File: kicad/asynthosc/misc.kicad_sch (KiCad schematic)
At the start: 8 parts, among them J4 LOUT, U4 TL074

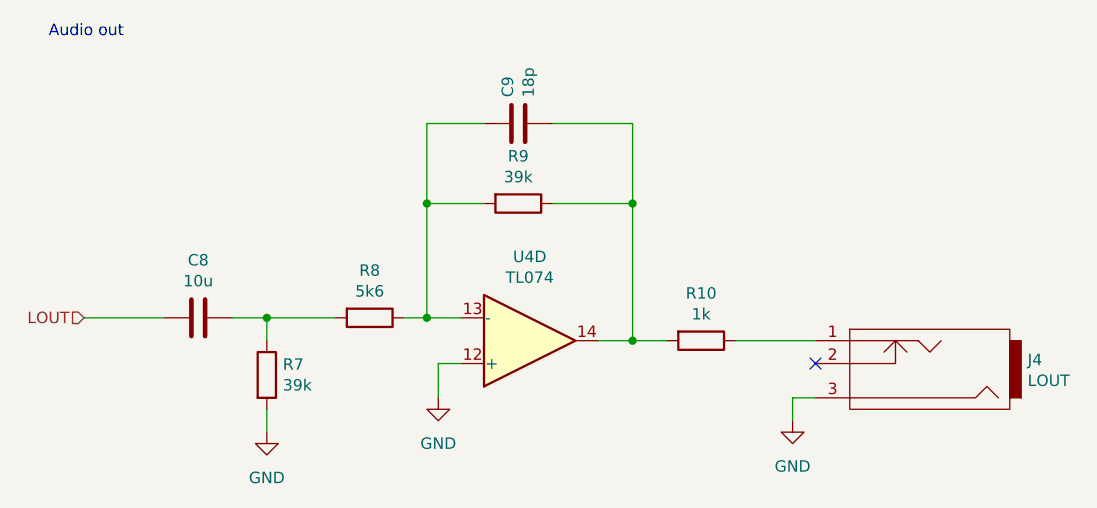
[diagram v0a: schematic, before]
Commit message: sch: wip, add .gitignore
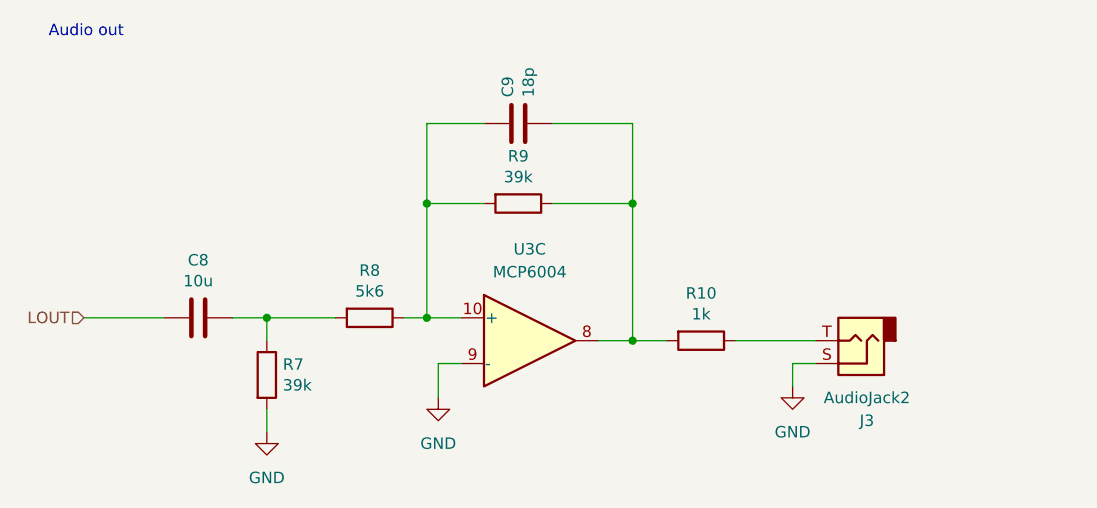
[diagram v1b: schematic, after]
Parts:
- removed J4: LOUT, connectors:THONKICONN, symbol jack_2p:JACK_2P
- removed U4: TL074, Package_SO:TSSOP-14_4.4x5mm_P0.65mm, symbol Amplifier_Operational:TL074
- added J3: AudioJack2, symbol Connector_Audio:AudioJack2
- added U3: MCP6004, symbol Amplifier_Operational:MCP6004
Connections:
- net GND: now also J3.S, U3.9 (-)
- net at C9.2, R10.2, R9.1: now also U3.8
- net at C9.1, R8.1, R9.2: now also U3.10 (+)
- net at R10.1: now also J3.T
- no-connect marks 1 -> 0
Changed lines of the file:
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@@
 		(color 0 0 0 0)
 	)
-	(no_connect
-		(at 115.57 54.61)
-	)
 	(wire
 		(pts
@@
 	(wire
 		(pts
-			(xy 115.57 58.42) (xy 113.03 58.42)
+			(xy 115.57 54.61) (xy 113.03 54.61)
 		)
 		(stroke
@@
 	(wire
 		(pts
-			(xy 113.03 58.42) (xy 113.03 60.96)
+			(xy 113.03 54.61) (xy 113.03 57.15)
 		)
 		(stroke
@@
 	)
 	(symbol
-		(lib_id "jack_2p:JACK_2P")
-		(at 127 54.61 180)
-		(unit 1)
-		(exclude_from_sim no)
-		(in_bom yes)
-		(on_board yes)
-		(dnp no)
-		(property "Reference" "J4"
-			(at 139.1412 54.2036 0)
-			(effects
-				(font
-					(size 1.27 1.27)
-				)
-				(justify right)
-			)
-		)
-		(property "Value" "LOUT"
-			(at 139.1412 56.515 0)
-			(effects
-				(font
-					(size 1.27 1.27)
-				)
-				(justify right)
-			)
-		)
-		(property "Footprint" "connectors:THONKICONN"
-			(at 127 54.61 0)
-			(effects
-				(font
-					(size 1.27 1.27)
-				)
-				(hide yes)
-			)
-		)
-		(property "Datasheet" ""
-			(at 127 54.61 0)
-			(effects
-				(font
-					(size 1.27 1.27)
-				)
-			)
-		)
-		(property "Description" ""
-			(at 127 54.61 0)
-			(effects
-				(font
-					(size 1.27 1.27)
-				)
-				(hide yes)
-			)
-		)
-		(pin "1"
-		)
-		(pin "2"
-		)
-		(pin "3"
-		)
-		(instances
-			(project "asynthosc"
-				(path "/d73e377a-a016-415f-8824-91cc6e4907b9/7d8430fa-40d5-422d-97f7-702a1a4b7211"
-					(reference "J4")
-					(unit 1)
-				)
-			)
-		)
-	)
-	(symbol
 		(lib_id "Device:R")
 		(at 102.87 52.07 270)
@@
 	(symbol
 		(lib_id "power:GND")
-		(at 113.03 60.96 0)
+		(at 113.03 57.15 0)
 		(unit 1)
 		(exclude_from_sim no)
@@
 		(fields_autoplaced yes)
 		(property "Reference" "#PWR025"
-			(at 113.03 67.31 0)
+			(at 113.03 63.5 0)
 			(effects
 				(font
@@
 		)
 		(property "Value" "GND"
-			(at 113.03 66.04 0)
+			(at 113.03 62.23 0)
 			(effects
 				(font
@@
 		)
 		(property "Footprint" ""
-			(at 113.03 60.96 0)
+			(at 113.03 57.15 0)
 			(effects
 				(font
@@
 		)
 		(property "Datasheet" ""
-			(at 113.03 60.96 0)
+			(at 113.03 57.15 0)
 			(effects
 				(font
@@
 		)
 		(property "Description" "Power symbol creates a global label with name \"GND\" , ground"
-			(at 113.03 60.96 0)
+			(at 113.03 57.15 0)
 			(effects
 				(font
@@
 	)
 	(symbol
+		(lib_id "Connector_Audio:AudioJack2")
+		(at 120.65 52.07 180)
+		(unit 1)
+		(exclude_from_sim no)
+		(in_bom yes)
+		(on_board yes)
+		(dnp no)
+		(property "Reference" "J3"
+			(at 121.285 60.96 0)
+			(effects
+				(font
+					(size 1.27 1.27)
+				)
+			)
+		)
+		(property "Value" "AudioJack2"
+			(at 121.285 58.42 0)
+			(effects
+				(font
+					(size 1.27 1.27)
+				)
+			)
+		)
+		(property "Footprint" ""
+			(at 120.65 52.07 0)
+			(effects
+				(font
+					(size 1.27 1.27)
+				)
+				(hide yes)
+			)
+		)
+		(property "Datasheet" "~"
+			(at 120.65 52.07 0)
+			(effects
+				(font
+					(size 1.27 1.27)
+				)
+				(hide yes)
+			)
+		)
+		(property "Description" "Audio Jack, 2 Poles (Mono / TS)"
+			(at 120.65 52.07 0)
+			(effects
+				(font
+					(size 1.27 1.27)
+				)
+				(hide yes)
+			)
+		)
+		(property "Sim.Device" "V"
+			(at 120.65 52.07 0)
+			(effects
+				(font
+					(size 1.27 1.27)
+				)
+				(hide yes)
+			)
+		)
+		(property "Sim.Type" "SIN"
+			(at 120.65 52.07 0)
+			(effects
+				(font
+					(size 1.27 1.27)
+				)
+				(hide yes)
+			)
+		)
+		(property "Sim.Pins" "S=- T=+"
+			(at 120.65 52.07 0)
+			(effects
+				(font
+					(size 1.27 1.27)
+				)
+				(hide yes)
+			)
+		)
+		(property "Sim.Params" "dc=0 ampl=0 f=1 td=0 theta=0 phase=0 ac=5"
+			(at 120.65 52.07 0)
+			(effects
+				(font
+					(size 1.27 1.27)
+				)
+				(hide yes)
+			)
+		)
+		(pin "S"
+		)
+		(pin "T"
+		)
+		(instances
+			(project "asynthosc"
+				(path "/d73e377a-a016-415f-8824-91cc6e4907b9/7d8430fa-40d5-422d-97f7-702a1a4b7211"
+					(reference "J3")
+					(unit 1)
+				)
+			)
+		)
+	)
+	(symbol
 		(lib_id "Device:R")
 		(at 66.04 49.53 270)
@@
 	)
 	(symbol
-		(lib_id "Amplifier_Operational:TL074")
-		(at 83.82 52.07 0)
-		(mirror x)
-		(unit 4)
-		(exclude_from_sim no)
-		(in_bom yes)
-		(on_board yes)
-		(dnp no)
-		(property "Reference" "U4"
-			(at 83.82 42.7482 0)
-			(effects
-				(font
-					(size 1.27 1.27)
-				)
-			)
-		)
-		(property "Value" "TL074"
-			(at 83.82 45.0596 0)
-			(effects
-				(font
-					(size 1.27 1.27)
-				)
-			)
-		)
-		(property "Footprint" "Package_SO:TSSOP-14_4.4x5mm_P0.65mm"
-			(at 82.55 54.61 0)
-			(effects
-				(font
-					(size 1.27 1.27)
-				)
-				(hide yes)
-			)
-		)
-		(property "Datasheet" "http://www.ti.com/lit/ds/symlink/tl071.pdf"
-			(at 85.09 57.15 0)
-			(effects
-				(font
-					(size 1.27 1.27)
-				)
-				(hide yes)
-			)
-		)
-		(property "Description" ""
-			(at 83.82 52.07 0)
-			(effects
-				(font
-					(size 1.27 1.27)
-				)
-				(hide yes)
-			)
-		)
-		(pin "1"
-		)
-		(pin "2"
-		)
-		(pin "3"
-		)
-		(pin "5"
-		)
-		(pin "6"
-		)
-		(pin "7"
-		)
-		(pin "10"
-		)
-		(pin "8"
-		)
-		(pin "9"
-		)
-		(pin "12"
-		)
-		(pin "13"
-		)
-		(pin "14"
-		)
-		(pin "11"
-		)
-		(pin "4"
-		)
-		(instances
-			(project "asynthosc"
-				(path "/d73e377a-a016-415f-8824-91cc6e4907b9/7d8430fa-40d5-422d-97f7-702a1a4b7211"
-					(reference "U4")
-					(unit 4)
-				)
-			)
-		)
-	)
-	(symbol
 		(lib_id "Device:C")
 		(at 46.99 49.53 270)
@@
 				)
 			)
+		)
+	)
+	(symbol
+		(lib_id "Amplifier_Operational:MCP6004")
+		(at 83.82 52.07 0)
+		(unit 3)
+		(exclude_from_sim no)
+		(in_bom yes)
+		(on_board yes)
+		(dnp no)
+		(fields_autoplaced yes)
+		(property "Reference" "U3"
+			(at 83.82 41.91 0)
+			(effects
+				(font
+					(size 1.27 1.27)
+				)
+			)
+		)
+		(property "Value" "MCP6004"
+			(at 83.82 44.45 0)
+			(effects
+				(font
+					(size 1.27 1.27)
+				)
+			)
+		)
+		(property "Footprint" ""
+			(at 82.55 49.53 0)
+			(effects
+				(font
+					(size 1.27 1.27)
+				)
+				(hide yes)
+			)
+		)
+		(property "Datasheet" "http://ww1.microchip.com/downloads/en/DeviceDoc/21733j.pdf"
+			(at 85.09 46.99 0)
+			(effects
+				(font
+					(size 1.27 1.27)
+				)
+				(hide yes)
+			)
+		)
+		(property "Description" "1MHz, Low-Power Op Amp, DIP-14/SOIC-14/TSSOP-14"
+			(at 83.82 52.07 0)
+			(effects
+				(font
+					(size 1.27 1.27)
+				)
+				(hide yes)
+			)
+		)
+		(property "Sim.Library" "/home/eve/Documents/asynth2osc/kicad/asynthosc/spice_mods/MCP600x.txt"
+			(at 83.82 52.07 0)
+			(effects
+				(font
+					(size 1.27 1.27)
+				)
+				(hide yes)
+			)
+		)
+		(property "Sim.Name" "MCP6004_pinout"
+			(at 83.82 52.07 0)
+			(effects
+				(font
+					(size 1.27 1.27)
+				)
+				(hide yes)
+			)
+		)
+		(property "Sim.Device" "SUBCKT"
+			(at 83.82 52.07 0)
+			(effects
+				(font
+					(size 1.27 1.27)
+				)
+				(hide yes)
+			)
+		)
+		(property "Sim.Pins" "1=1 2=2 3=3 4=4 5=5 6=6 7=7 8=8 9=9 10=10 11=11 12=12 13=13 14=14"
+			(at 83.82 52.07 0)
+			(effects
+				(font
+					(size 1.27 1.27)
+				)
+				(hide yes)
+			)
+		)
+		(pin "1"
+		)
+		(pin "8"
+		)
+		(pin "11"
+		)
+		(pin "9"
+		)
+		(pin "4"
+		)
+		(pin "2"
+		)
+		(pin "5"
+		)
+		(pin "6"
+		)
+		(pin "3"
+		)
+		(pin "10"
+		)
+		(pin "12"
+		)
+		(pin "14"
+		)
+		(pin "7"
+		)
+		(pin "13"
+		)
+		(instances
+			(project "asynthosc"
+				(path "/d73e377a-a016-415f-8824-91cc6e4907b9/7d8430fa-40d5-422d-97f7-702a1a4b7211"
+					(reference "U3")
+					(unit 3)
+				)
+			)
